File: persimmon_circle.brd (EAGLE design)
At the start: 35 x 55 mm, 34 parts

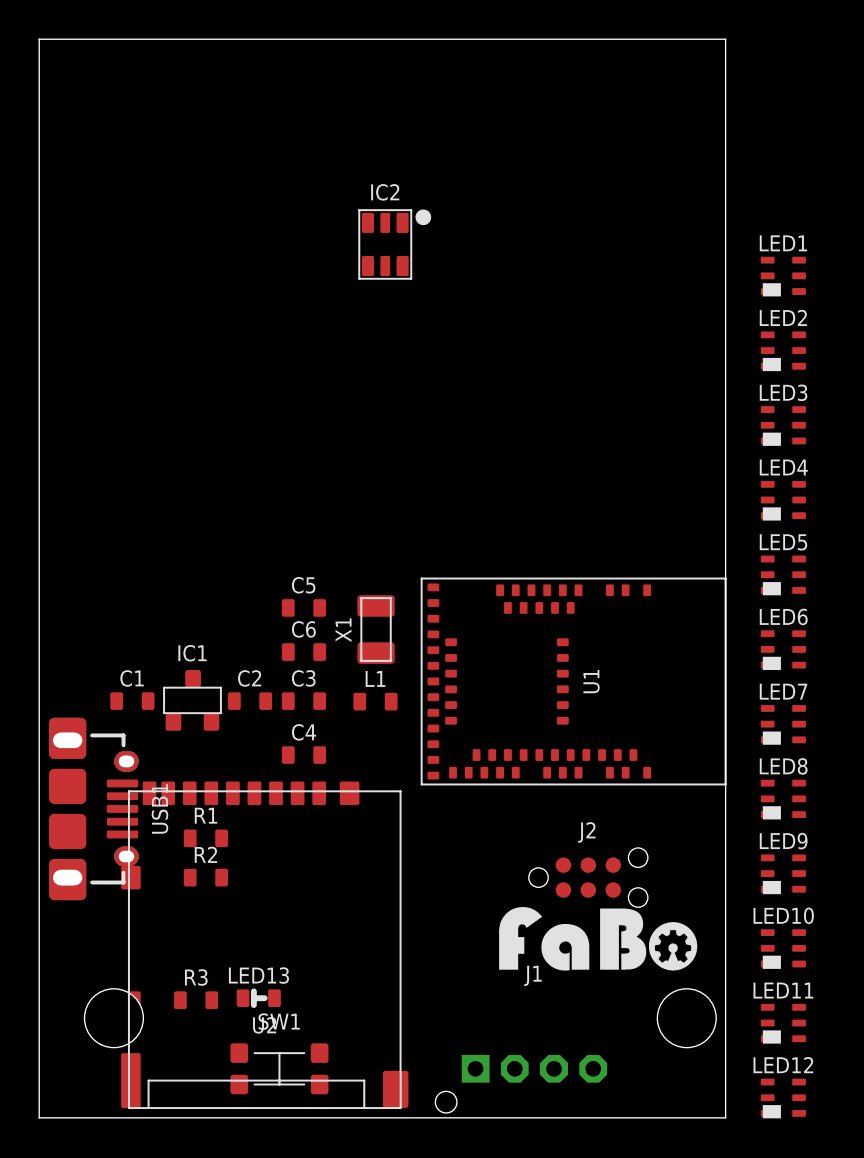
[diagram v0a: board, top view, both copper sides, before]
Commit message: Persimmon circle Rev.Beta1　リファイン
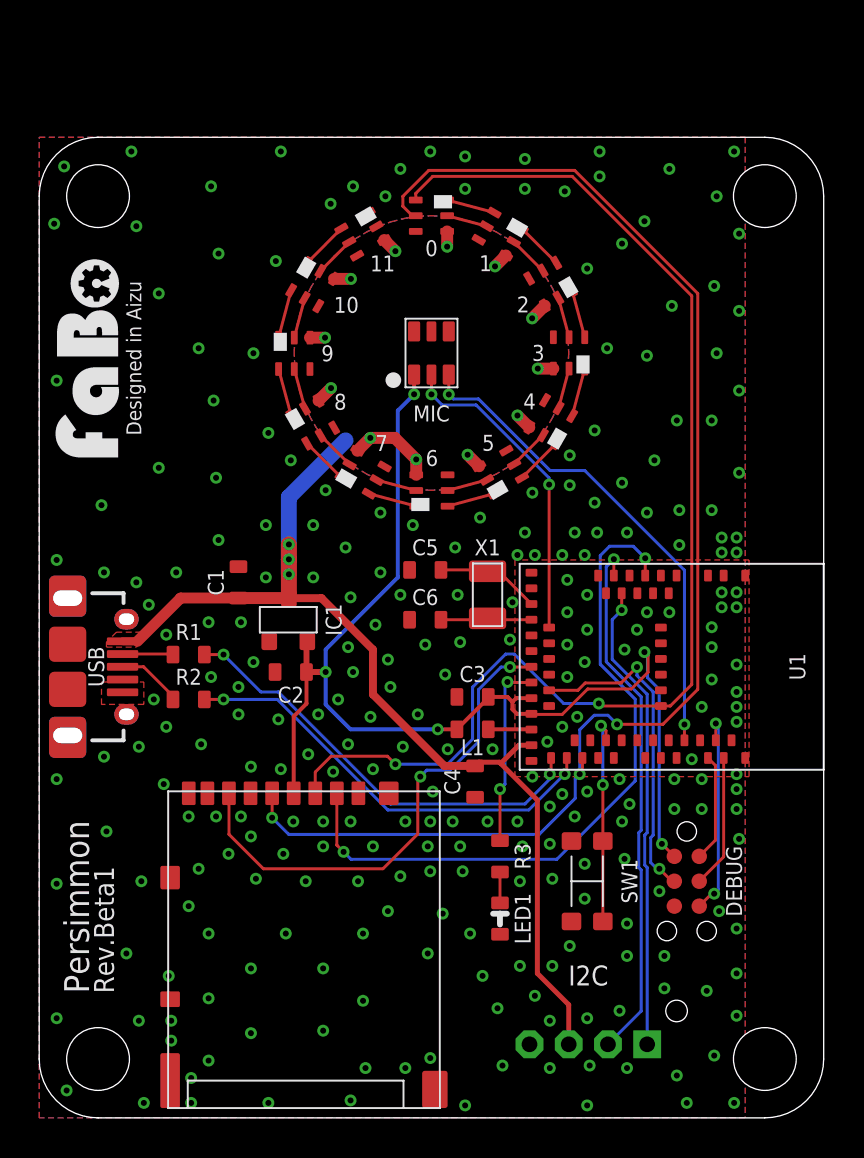
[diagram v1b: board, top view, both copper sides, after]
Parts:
- removed IC2: (no value), FaBo-Sound:ICS41351
- removed J1: (no value), FaBo-Template:FABO_BRICK_I2C_B04B-PASK-1
- removed J2: (no value), FaBo-Debbuger:TC2030-IDC-NL
- removed LED10, LED11, LED12, LED2, LED3, LED4, LED5, LED6, LED7, LED8, LED9: (no value), FaBo-LED:APA102_2020
- removed LED13: (no value), FaBo-LED:0603
- removed USB1: (no value), FaBo-USB:ZX62D-B-5PA8
- added 0, 1, 10, 11, 2, 3, 4, 5, 6, 7, 8, 9: (no value), FaBo-LED:APA102_2020
- added DEBUG: (no value), FaBo-Debbuger:TC2030-IDC-NL
- added I2C: (no value), FaBo-Template:FABO_BRICK_I2C_B04B-PASK-1
- added MIC: (no value), FaBo-Sound:ICS41351
- added USB: (no value), FaBo-USB:ZX62D-B-5PA8
- LED1: device FaBo-LED:APA102_2020 -> FaBo-LED:0603
- moved LOGO2 39.7 mm to (4.45, 38.7), turned to 90 degrees
- moved LED1 35.8 mm to (23.5, 10.2), turned to 270 degrees
- moved SW1 18.4 mm to (27.9, 12.1), turned to 270 degrees
- moved R3 17.1 mm to (23.5, 13.3), turned to 90 degrees
- moved R1 9.41 mm to (7.62, 23.6)
- moved R2 9.13 mm to (7.62, 21.3)
- moved C4 8.83 mm to (22.2, 17.1), turned to 90 degrees
- moved C3 8.60 mm to (22.1, 21.5)
- moved C1 8.12 mm to (10.2, 27.3), turned to 270 degrees
- moved C5 6.48 mm to (19.7, 27.9)
- moved C6 6.40 mm to (19.7, 25.4)
- moved IC1 6.39 mm to (12.7, 25.4)
- moved X1 5.95 mm to (22.9, 26.7)
- moved L1 5.15 mm to (22.1, 19.8)
- moved U1 5.06 mm to (32.2, 23.0)
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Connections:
- net N$3 renamed X2
- net N$4 renamed X1
- net N$5 renamed L1
- removed net N$1: R1.1, USB1.2
- removed net N$10: LED1.CKO, LED2.CKI
- removed net N$11: LED2.SDO, LED3.SDI
- removed net N$12: LED2.CKO, LED3.CKI
- removed net N$13: LED3.SDO, LED4.SDI
- removed net N$14: LED3.CKO, LED4.CKI
- removed net N$15: LED4.SDO, LED5.SDI
- removed net N$16: LED4.CKO, LED5.CKI
- removed net N$17: LED5.SDO, LED6.SDI
- removed net N$18: LED5.CKO, LED6.CKI
- removed net N$19: LED7.SDO, LED8.SDI
- removed net N$2: R2.1, USB1.3
- removed net N$20: LED7.CKO, LED8.CKI
- removed net N$21: LED8.SDO, LED9.SDI
- removed net N$22: LED8.CKO, LED9.CKI
- removed net N$23: LED10.SDI, LED9.SDO
- removed net N$24: LED10.CKI, LED9.CKO
- removed net N$25: LED10.SDO, LED11.SDI
- removed net N$26: LED10.CKO, LED11.CKI
- removed net N$27: LED11.SDO, LED12.SDI
- removed net N$28: LED11.CKO, LED12.CKI
- removed net N$6: LED13.ANODE, R3.1
- removed net N$9: LED1.SDO, LED2.SDI
- new net CI0: 0.CKO, 1.CKI
- new net CI1: 1.CKO, 2.CKI
- new net CI10: 10.CKO, 11.CKI
- new net CI2: 2.CKO, 3.CKI
- new net CI3: 3.CKO, 4.CKI
- new net CI4: 4.CKO, 5.CKI
- new net CI6: 6.CKO, 7.CKI
- new net CI7: 7.CKO, 8.CKI
- new net CI8: 8.CKO, 9.CKI
- new net CI9: 10.CKI, 9.CKO
- new net DI0: 0.SDO, 1.SDI
- new net DI1: 1.SDO, 2.SDI
- new net DI10: 10.SDO, 11.SDI
- new net DI2: 2.SDO, 3.SDI
- new net DI3: 3.SDO, 4.SDI
- new net DI4: 4.SDO, 5.SDI
- new net DI6: 6.SDO, 7.SDI
- new net DI7: 7.SDO, 8.SDI
- new net DI8: 8.SDO, 9.SDI
- new net DI9: 10.SDI, 9.SDO
- new net LED1: LED1.ANODE, R3.1
- new net USB_DM: R1.1, USB.2
- new net USB_DP: R2.1, USB.3
- net 3V3: now also DEBUG.1, MIC.1; no longer IC2.1, J2.1
- net 5V: now also 0.VCC, 1.VCC, 10.VCC, 11.VCC, 2.VCC, 3.VCC, 4.VCC, 5.VCC, 6.VCC, 7.VCC, 8.VCC, 9.VCC, I2C.VCC, USB.1; no longer J1.VCC, LED1.VCC, LED10.VCC, LED11.VCC, LED12.VCC, LED2.VCC, LED3.VCC, LED4.VCC, LED5.VCC, LED6.VCC, LED7.VCC, LED8.VCC, LED9.VCC, USB1.1
- net CI_1: now also 5.CKO, 6.CKI; no longer LED6.CKO, LED7.CKI
- net DI_1: now also 5.SDO, 6.SDI; no longer LED6.SDO, LED7.SDI
- net GND: now also 0.GND, 1.GND, 10.GND, 11.GND, 2.GND, 3.GND, 4.GND, 5.GND, 6.GND, 7.GND, 8.GND, 9.GND, DEBUG.5, I2C.GND, LED1.CATHODE, MIC.4, MIC.5, MIC.6, USB.5; no longer IC2.4, IC2.5, IC2.6, J1.GND, J2.5, LED1.GND, LED10.GND, LED11.GND, LED12.GND, LED13.CATHODE, LED2.GND, LED3.GND, LED4.GND, LED5.GND, LED6.GND, LED7.GND, LED8.GND, LED9.GND, USB1.5
- net MOSI: now also 0.SDI; no longer LED1.SDI
- net P0.09: now also DEBUG.6; no longer J2.6
- net P0.11: now also DEBUG.3; no longer J2.3
- net PDMCLK: now also MIC.2; no longer IC2.2
- net PDMDIN: now also MIC.3; no longer IC2.3
- net SCK: now also 0.CKI; no longer LED1.CKI
- net SCL: now also I2C.SCL; no longer J1.SCL
- net SDA: now also I2C.SDA; no longer J1.SDA
- net SWCLK: now also DEBUG.4; no longer J2.4
- net SWDIO: now also DEBUG.2; no longer J2.2
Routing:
- net SCK: track 0.00 -> 69.3 mm, vias 0 -> 3
- net 5V: track 0.00 -> 66.5 mm, vias 0 -> 15
- net MOSI: track 0.00 -> 63.3 mm, vias 0 -> 2
- net 3V3: track 0.00 -> 60.1 mm, vias 0 -> 5
- net D4: track 0.00 -> 35.7 mm, vias 0 -> 2
- net SDA: track 0.00 -> 27.3 mm, vias 0 -> 1
- net MISO: track 0.00 -> 25.7 mm, vias 0 -> 2
- net PDMDIN: track 0.00 -> 25.4 mm, vias 0 -> 2
- net SCL: track 0.00 -> 24.0 mm, vias 0 -> 1
- net D-: track 0.00 -> 22.4 mm, vias 0 -> 2
- net D+: track 0.00 -> 22.3 mm, vias 0 -> 2
- net P0.11: track 0.00 -> 16.9 mm, vias 0 -> 2
- net PDMCLK: track 0.00 -> 16.4 mm, vias 0 -> 2
- net RESET: track 0.00 -> 10.9 mm, vias 0 -> 2
- net P0.09: track 0.00 -> 10.7 mm, vias 0 -> 2
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- added copper zone on layer 1, net 5V
- added copper zone on layer 16, net 5V
- added copper zone on layer 1, net GND
- added copper zone on layer 16, net GND
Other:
- board size 35 x 55 mm -> 40 x 50 mm
- board text added: "Designed in Aizu"
- board text added: "Persimmon"
- board text added: "Rev.Beta1"
